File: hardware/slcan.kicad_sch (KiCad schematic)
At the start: 1 part, among them SW1 SW_DPST

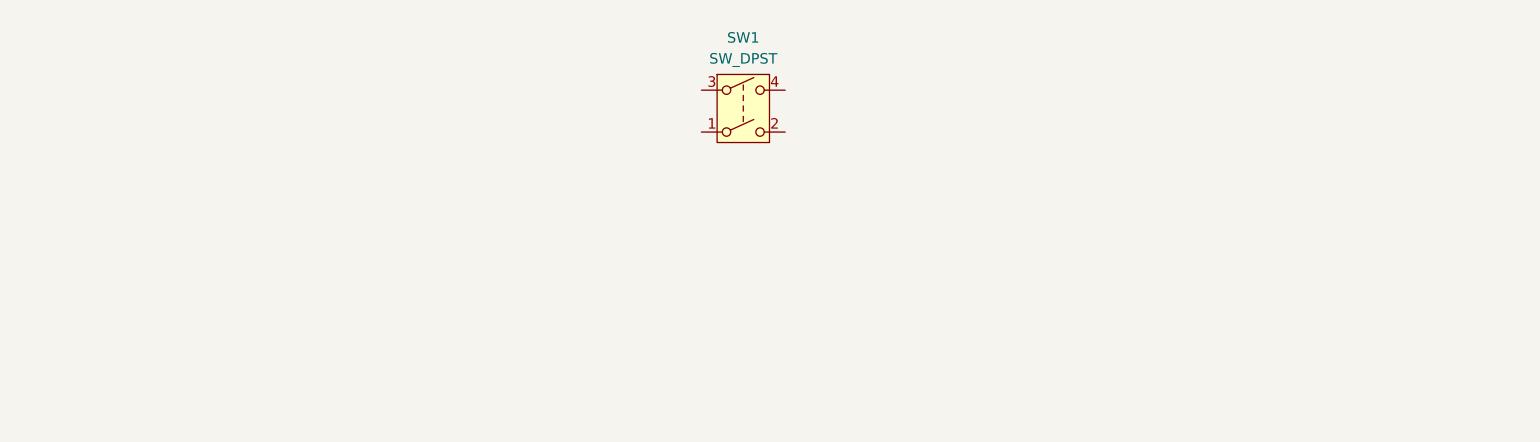
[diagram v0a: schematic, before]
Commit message: V1.0
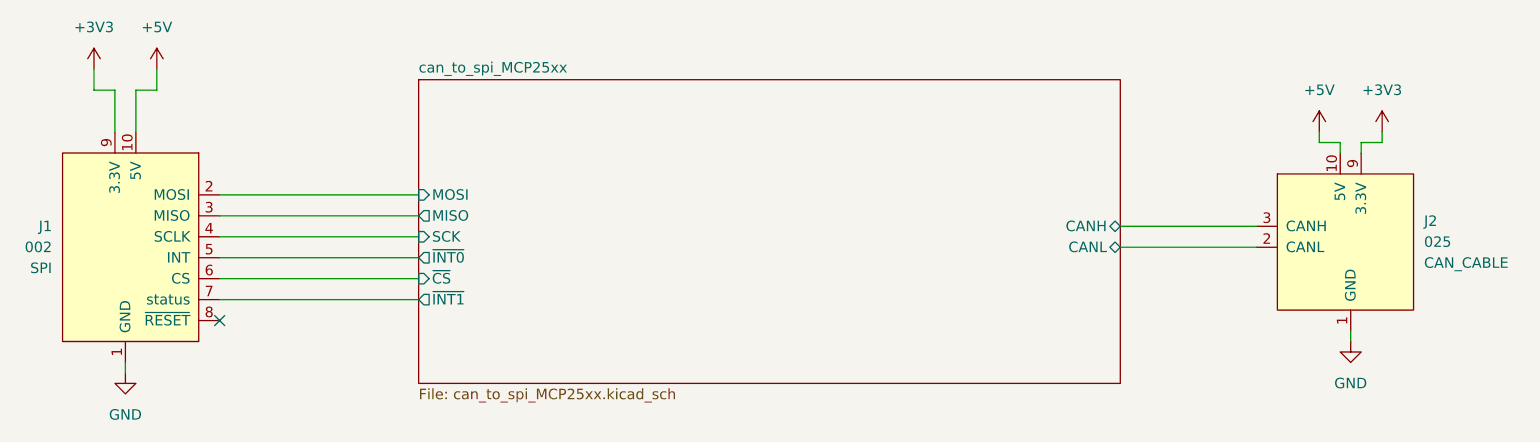
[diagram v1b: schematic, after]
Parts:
- removed SW1: SW_DPST, symbol Switch:SW_DPST
- added J1: 002, put_on_edge:on_edge_2x05_device, symbol put_on_edge_local:002_SPI_device
- added J2: 025, put_on_edge:on_edge_2x05_host, symbol put_on_edge_local:025_CAN_cable_host
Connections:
- new net +3V3: J1.9 (3.3V), J2.9 (3.3V)
- new net +5V: J1.10 (5V), J2.10 (5V)
- new net GND: J1.1 (GND), J2.1 (GND)
- new net can_to_spi_MCP25xx/CANH: J2.3 (CANH)
- new net can_to_spi_MCP25xx/CANL: J2.2 (CANL)
- new net can_to_spi_MCP25xx/MISO: J1.3 (MISO)
- new net can_to_spi_MCP25xx/MOSI: J1.2 (MOSI)
- new net can_to_spi_MCP25xx/SCK: J1.4 (SCLK)
- new net can_to_spi_MCP25xx/~{CS}: J1.6 (CS)
- new net can_to_spi_MCP25xx/~{INT0}: J1.5 (INT)
- new net can_to_spi_MCP25xx/~{INT1}: J1.7 (status)
- no-connect marks 0 -> 1
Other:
- added sheet can_to_spi_MCP25xx (can_to_spi_MCP25xx.kicad_sch)
